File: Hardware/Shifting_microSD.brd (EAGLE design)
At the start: 20.4 x 24.6 mm, 21 parts, among them J1 USD_CONNECTOR, Q1 200mA/50V, Q2 200mA/50V, Q3 200mA/50V, Q4 200mA/50V, U2 3.3V

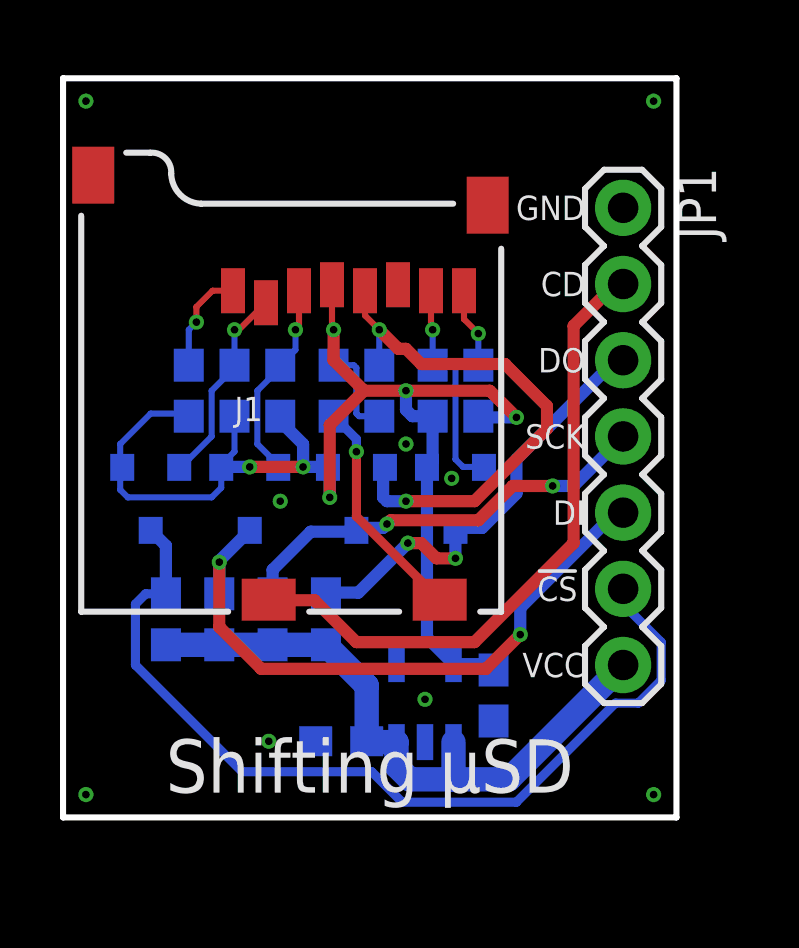
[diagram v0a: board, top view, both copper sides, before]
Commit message: Initial design finished
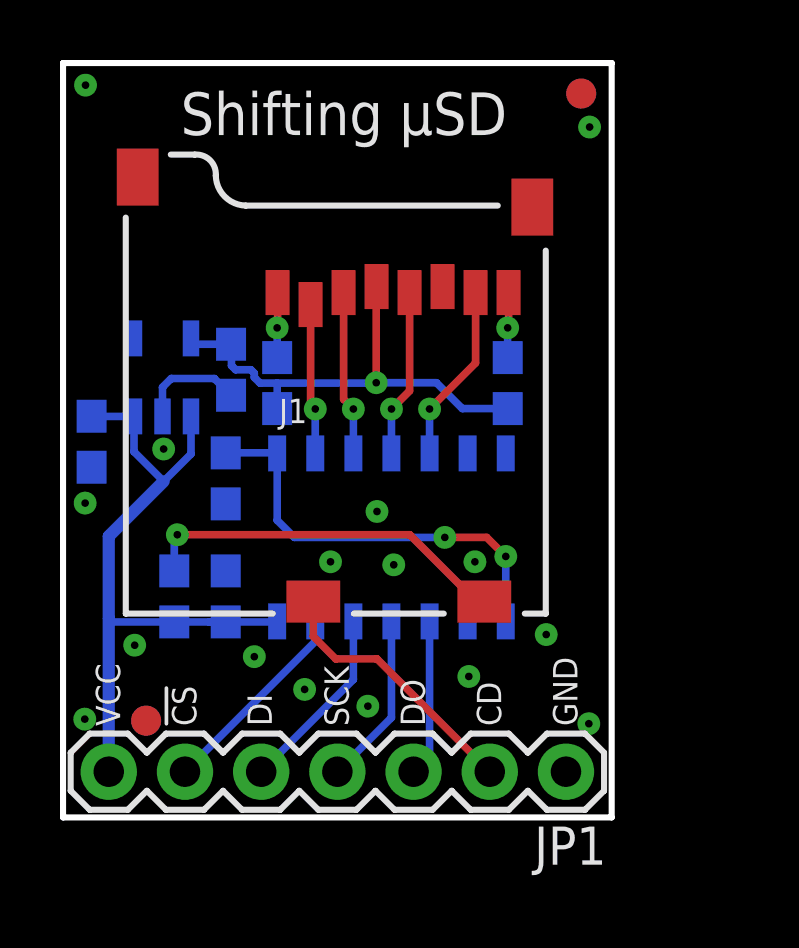
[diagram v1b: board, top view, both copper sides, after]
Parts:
- removed Q1, Q2, Q3, Q4: 200mA/50V, SparkFun-DiscreteSemi:SOT23-3
- removed R10, R11, R4, R5, R6, R7, R8, R9: 10K, SparkFun-Resistors:0603-RES
- added C3, C4: 0.1uF, SparkFun-Capacitors:0603-CAP
- added FID1, FID2, FID3, FID4: FIDUCIAL1X2, SparkFun-Aesthetics:FIDUCIAL-1X2
- added LOGO1: SFE_LOGO_FLAME.3_INCH, SparkFun-Aesthetics:SFE_LOGO_FLAME_.3
- added LOGO2: OSHW-LOGOS, SparkFun-Aesthetics:OSHW-LOGO-S
- added U1: (no value), SparkFun-DigitalIC:SO14
- moved JP1 18.9 mm to (16.8, 1.52), turned to 180 degrees
- moved C2 13.9 mm to (5.60, 14.9)
- moved U2 13.9 mm to (3.31, 14.7)
- moved C1 13.0 mm to (0.95, 12.5), turned to 270 degrees
- moved R3 8.67 mm to (3.71, 7.37), turned to 270 degrees
- moved R1 2.96 mm to (7.14, 14.5)
- moved J1 1.49 mm to (16.1, 6.79)
- moved R2 1.01 mm to (14.8, 14.5)
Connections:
- removed net !CS: J1.CS, Q4.2, R10.1
- removed net N$2: JP1.5, Q3.3, R9.1
- removed net N$5: JP1.4, Q2.3, R7.1
- removed net N$7: JP1.3, Q1.3, R5.1
- removed net SCK: J1.SCLK, Q2.2, R6.1
- removed net VCC: C1.1, JP1.7, R11.2, R5.2, R7.2, R9.2, U2.1, U2.3
- new net !CS_3V3: J1.CS, U1.2
- new net 3.3V: C4.1, U1.1, U1.8
- new net DI_3V3: J1.DI, U1.3
- new net DO_3V3: J1.DO, U1.5
- new net N$3: JP1.4, U1.11
- new net SCK_3V3: J1.SCLK, U1.4
- new net VDD_IO: C1.1, C3.1, JP1.7, R3.2, U1.14, U2.1, U2.3
- net 3V3: no longer Q1.1, Q2.1, Q3.1, Q4.1, R10.2, R3.2, R4.2, R6.2, R8.2
- net DI: now also JP1.5, U1.12; no longer J1.DI, Q3.2, R8.1
- net DO: now also JP1.3, U1.10; no longer J1.DO, Q1.2, R4.1
- net GND: now also C3.2, C4.2, U1.7
- net N$1: now also U1.13; no longer Q4.3, R11.1
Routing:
- net 3V3: track 48.5 -> 16.1 mm, vias 6 -> 1
- net N$1: track 30.2 -> 6.81 mm
- net VDD_IO: track 0.00 -> 22.6 mm
- net VCC: track 21.5 -> 0.00 mm
- net N$2: track 21.4 -> 0.00 mm, vias 2 -> 0
- net SCK: track 17.6 -> 0.00 mm, vias 2 -> 0
- net N$7: track 15.1 -> 0.00 mm, vias 2 -> 0
- net N$5: track 14.7 -> 0.00 mm, vias 2 -> 0
- net 3.3V: track 0.00 -> 14.2 mm, vias 0 -> 2
- net CD: track 21.6 -> 8.91 mm
- net !CS: track 7.18 -> 0.00 mm, vias 1 -> 0
- net DO_3V3: track 0.00 -> 6.00 mm, vias 0 -> 1
- net N$3: track 0.00 -> 5.76 mm
- net SCK_3V3: track 0.00 -> 5.61 mm, vias 0 -> 1
- net DI_3V3: track 0.00 -> 5.50 mm, vias 0 -> 1
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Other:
- board size 20.4 x 24.6 mm -> 18.3 x 25.1 mm
